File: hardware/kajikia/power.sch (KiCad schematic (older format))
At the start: 80 parts, among them J39 Screw_Terminal_01x02, J40 Conn_01x01, J41 Conn_01x01, J42 Conn_01x01, J43 Conn_01x01, J44 Conn_01x01, J45 Conn_01x01, J46 Conn_01x01, J47 Conn_01x01, J48 Conn_01x01, J49 Conn_01x01, J50 Conn_01x01, J51 Conn_01x01, J52 Conn_01x01, J53 Conn_01x01, J54 Conn_01x01, J55 Conn_01x01, J56 Conn_01x01, J57 Conn_01x01, J58 Conn_01x01, J59 Conn_01x01, Q1 AON6144, U2 LM1117-3.3, U3 AOZ1284, U4 AOZ1284

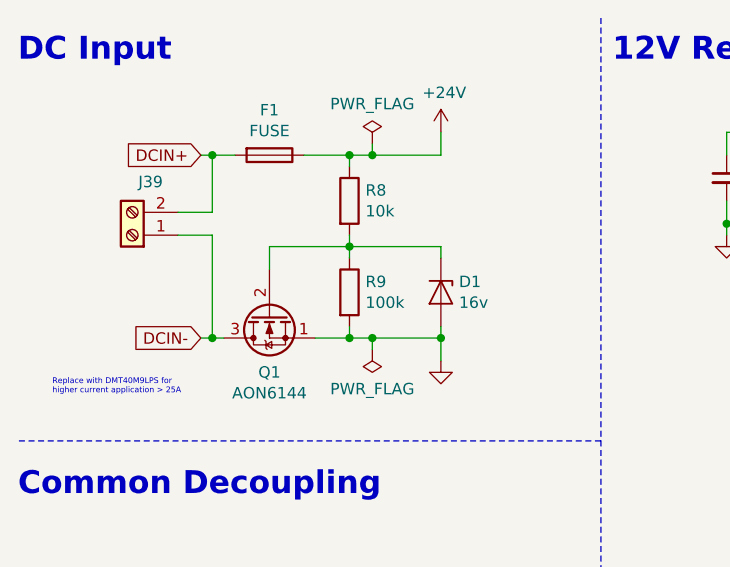
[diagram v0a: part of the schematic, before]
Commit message: fuses
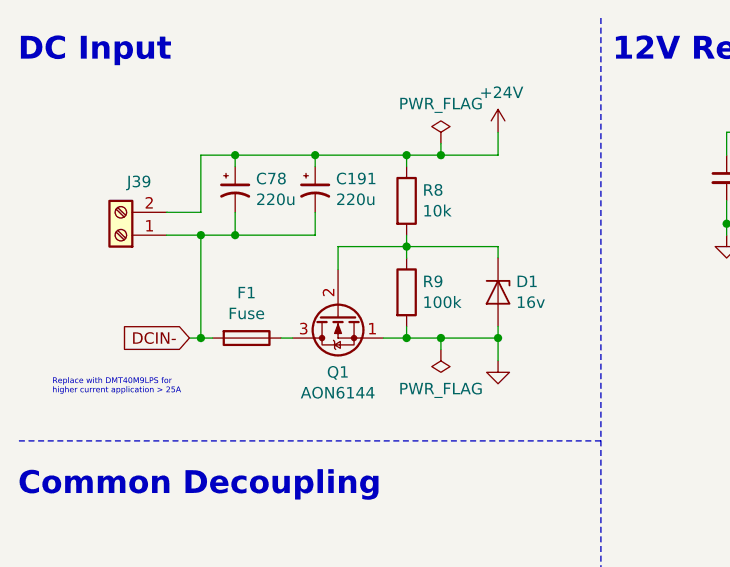
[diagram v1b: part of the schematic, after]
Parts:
- added C191, C78: 220u, Capacitor_SMD:CP_Elec_6.3x7.7, symbol Device:CP1_Small
- F1: value FUSE -> Fuse
- JP14: footprint (none) -> _Generic:Solder Jumper 2P
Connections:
- net +24V: now also J39.2 (Pin_2), C191.1, C78.1; no longer F1.1
- net DCIN-: now also F1.2, C191.2, C78.2; no longer Q1.3 (D)
- removed net DCIN+: F1.2, J39.2 (Pin_2)
- new net: F1.1, Q1.3 (D)
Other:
- moved on the sheet: D1, J39, Q1, R8, R9
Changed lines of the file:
@@
 L power:+24V #PWR017
 U 1 1 5C334E02
-P 2400 1050
-F 0 "#PWR017" H 2400 900 50  0001 C CNN
-F 1 "+24V" H 2415 1223 50  0000 C CNN
-F 2 "" H 2400 1050 50  0001 C CNN
-F 3 "" H 2400 1050 50  0001 C CNN
-	1    2400 1050
-	1    0    0    -1
-$EndComp
-Wire Wire Line
-	1250 1500 1400 1500
-Wire Wire Line
-	1400 1500 1400 1950
-Wire Wire Line
-	1250 1400 1400 1400
-Wire Wire Line
-	1400 1400 1400 1150
+P 2650 1050
+F 0 "#PWR017" H 2650 900 50  0001 C CNN
+F 1 "+24V" H 2665 1223 50  0000 C CNN
+F 2 "" H 2650 1050 50  0001 C CNN
+F 3 "" H 2650 1050 50  0001 C CNN
+	1    2650 1050
+	1    0    0    -1
+$EndComp
+Wire Wire Line
+	1200 1500 1350 1500
+Wire Wire Line
+	1200 1400 1350 1400
 $Comp
 L #Power:GND #PWR018
 U 1 1 5C34B6E8
-P 2400 2050
-F 0 "#PWR018" H 2400 1800 50  0001 C CNN
-F 1 "GND" H 2400 1900 50  0001 C CNN
-F 2 "" H 2400 2050 50  0001 C CNN
-F 3 "" H 2400 2050 50  0001 C CNN
-	1    2400 2050
-	1    0    0    -1
-$EndComp
-Wire Wire Line
-	2400 1950 2400 2050
-Wire Wire Line
-	2400 1050 2400 1150
-Wire Wire Line
-	1400 1150 1500 1150
-$Comp
-L Device:Fuse F1
-U 1 1 5C35C7B9
-P 1650 1150
-F 0 "F1" V 1453 1150 50  0000 C CNN
-F 1 "FUSE" V 1544 1150 50  0000 C CNN
-F 2 "_Generic:SMD_Fuseholder" V 1580 1150 50  0001 C CNN
-F 3 "~" H 1650 1150 50  0001 C CNN
-	1    1650 1150
-	0    1    1    0
-$EndComp
+P 2650 2050
+F 0 "#PWR018" H 2650 1800 50  0001 C CNN
+F 1 "GND" H 2650 1900 50  0001 C CNN
+F 2 "" H 2650 2050 50  0001 C CNN
+F 3 "" H 2650 2050 50  0001 C CNN
+	1    2650 2050
+	1    0    0    -1
+$EndComp
+Wire Wire Line
+	2650 1950 2650 2050
+Wire Wire Line
+	2650 1050 2650 1150
 $Comp
 L power:+12V #PWR034
@@
 F 0 "JP14" H 8300 1363 50  0000 C CNN
 F 1 "SolderJumper_2_Open" H 8300 1250 50  0001 C CNN
-F 2 "" H 8300 1250 50  0001 C CNN
+F 2 "_Generic:Solder Jumper 2P" H 8300 1250 50  0001 C CNN
 F 3 "~" H 8300 1250 50  0001 C CNN
 	1    8300 1250
@@
 Power LED
 Wire Wire Line
-	1400 1950 1450 1950
+	1350 1950 1400 1950
 $Comp
 L Device:Q_NMOS_SGD Q1
 U 1 1 5C3AA6BF
-P 1650 1850
-F 0 "Q1" V 1900 1850 50  0000 C CNN
-F 1 "AON6144" V 1991 1850 50  0000 C CNN
-F 2 "_Generic:DFN5x6-8" H 1850 1950 50  0001 C CNN
-F 3 "~" H 1650 1850 50  0001 C CNN
-	1    1650 1850
+P 1950 1850
+F 0 "Q1" V 2200 1850 50  0000 C CNN
+F 1 "AON6144" V 2291 1850 50  0000 C CNN
+F 2 "_Generic:DFN5x6-8" H 2150 1950 50  0001 C CNN
+F 3 "~" H 1950 1850 50  0001 C CNN
+	1    1950 1850
 	0    -1   1    0
 $EndComp
 Wire Wire Line
-	1850 1950 2000 1950
+	2150 1950 2250 1950
 $Comp
 L Device:R R8
 U 1 1 5C407302
-P 2000 1350
-F 0 "R8" H 2070 1396 50  0000 L CNN
-F 1 "10k" H 2070 1305 50  0000 L CNN
-F 2 "_Generic:0603_RES" V 1930 1350 50  0001 C CNN
-F 3 "~" H 2000 1350 50  0001 C CNN
-	1    2000 1350
+P 2250 1350
+F 0 "R8" H 2320 1396 50  0000 L CNN
+F 1 "10k" H 2320 1305 50  0000 L CNN
+F 2 "_Generic:0603_RES" V 2180 1350 50  0001 C CNN
+F 3 "~" H 2250 1350 50  0001 C CNN
+	1    2250 1350
 	1    0    0    -1
 $EndComp
@@
 L Device:D_Zener D1
 U 1 1 5C407892
-P 2400 1750
-F 0 "D1" V 2354 1829 50  0000 L CNN
-F 1 "16v" V 2445 1829 50  0000 L CNN
-F 2 "_Generic:SOD-523_DIODE" H 2400 1750 50  0001 C CNN
-F 3 "~" H 2400 1750 50  0001 C CNN
-	1    2400 1750
+P 2650 1750
+F 0 "D1" V 2604 1829 50  0000 L CNN
+F 1 "16v" V 2695 1829 50  0000 L CNN
+F 2 "_Generic:SOD-523_DIODE" H 2650 1750 50  0001 C CNN
+F 3 "~" H 2650 1750 50  0001 C CNN
+	1    2650 1750
 	0    1    1    0
 $EndComp
 Wire Wire Line
-	2400 1600 2400 1550
-Wire Wire Line
-	2400 1550 2000 1550
-Wire Wire Line
-	1650 1550 1650 1650
-Wire Wire Line
-	2000 1550 2000 1500
-Wire Wire Line
-	2400 1900 2400 1950
-Connection ~ 2400 1950
+	2650 1600 2650 1550
+Wire Wire Line
+	2650 1550 2250 1550
+Wire Wire Line
+	1950 1550 1950 1650
+Wire Wire Line
+	2250 1550 2250 1500
+Wire Wire Line
+	2650 1900 2650 1950
+Connection ~ 2650 1950
 $Comp
 L Device:R R9
 U 1 1 5C479547
-P 2000 1750
-F 0 "R9" H 2070 1796 50  0000 L CNN
-F 1 "100k" H 2070 1705 50  0000 L CNN
-F 2 "_Generic:0603_RES" V 1930 1750 50  0001 C CNN
-F 3 "~" H 2000 1750 50  0001 C CNN
-	1    2000 1750
-	1    0    0    -1
-$EndComp
-Wire Wire Line
-	2000 1900 2000 1950
-Connection ~ 2000 1950
-Wire Wire Line
-	2000 1950 2100 1950
-Wire Wire Line
-	2000 1600 2000 1550
-Connection ~ 2000 1550
-Wire Wire Line
-	2000 1550 1650 1550
+P 2250 1750
+F 0 "R9" H 2320 1796 50  0000 L CNN
+F 1 "100k" H 2320 1705 50  0000 L CNN
+F 2 "_Generic:0603_RES" V 2180 1750 50  0001 C CNN
+F 3 "~" H 2250 1750 50  0001 C CNN
+	1    2250 1750
+	1    0    0    -1
+$EndComp
+Wire Wire Line
+	2250 1900 2250 1950
+Connection ~ 2250 1950
+Wire Wire Line
+	2250 1600 2250 1550
+Connection ~ 2250 1550
+Wire Wire Line
+	2250 1550 1950 1550
 Text Notes 700  2200 0    25   ~ 0
 Replace with DMT40M9LPS for\nhigher current application > 25A
@@
 L power:PWR_FLAG #FLG07
 U 1 1 5C5382D5
-P 2100 2000
-F 0 "#FLG07" H 2100 2075 50  0001 C CNN
-F 1 "PWR_FLAG" H 2100 2173 50  0000 C CNN
-F 2 "" H 2100 2000 50  0001 C CNN
-F 3 "~" H 2100 2000 50  0001 C CNN
-	1    2100 2000
+P 2400 2000
+F 0 "#FLG07" H 2400 2075 50  0001 C CNN
+F 1 "PWR_FLAG" H 2400 2173 50  0000 C CNN
+F 2 "" H 2400 2000 50  0001 C CNN
+F 3 "~" H 2400 2000 50  0001 C CNN
+	1    2400 2000
 	-1   0    0    1
 $EndComp
 Wire Wire Line
-	2100 2000 2100 1950
-Connection ~ 2100 1950
-Wire Wire Line
-	2100 1950 2400 1950
+	2400 2000 2400 1950
 $Comp
 L power:PWR_FLAG #FLG06
 U 1 1 5C5499F4
-P 2100 1100
-F 0 "#FLG06" H 2100 1175 50  0001 C CNN
-F 1 "PWR_FLAG" H 2100 1274 50  0000 C CNN
-F 2 "" H 2100 1100 50  0001 C CNN
-F 3 "~" H 2100 1100 50  0001 C CNN
-	1    2100 1100
-	1    0    0    -1
-$EndComp
-Wire Wire Line
-	2100 1100 2100 1150
-Connection ~ 2100 1150
-Wire Wire Line
-	2100 1150 2400 1150
-Wire Wire Line
-	2000 1200 2000 1150
-Connection ~ 2000 1150
-Wire Wire Line
-	2000 1150 2100 1150
-Wire Wire Line
-	1800 1150 2000 1150
+P 2400 1100
+F 0 "#FLG06" H 2400 1175 50  0001 C CNN
+F 1 "PWR_FLAG" H 2400 1274 50  0000 C CNN
+F 2 "" H 2400 1100 50  0001 C CNN
+F 3 "~" H 2400 1100 50  0001 C CNN
+	1    2400 1100
+	1    0    0    -1
+$EndComp
+Wire Wire Line
+	2400 1100 2400 1150
+Wire Wire Line
+	2250 1200 2250 1150
+Connection ~ 2250 1150
 $Comp
 L Connector:Screw_Terminal_01x02 J39
 U 1 1 5C365574
-P 1050 1500
-F 0 "J39" H 970 1267 50  0000 C CNN
-F 1 "Screw_Terminal_01x02" H 970 1266 50  0001 C CNN
-F 2 "_Generic:KF635-2P" H 1050 1500 50  0001 C CNN
-F 3 "~" H 1050 1500 50  0001 C CNN
-	1    1050 1500
+P 1000 1500
+F 0 "J39" H 920 1267 50  0000 C CNN
+F 1 "Screw_Terminal_01x02" H 920 1266 50  0001 C CNN
+F 2 "_Generic:KF635-2P" H 1000 1500 50  0001 C CNN
+F 3 "~" H 1000 1500 50  0001 C CNN
+	1    1000 1500
 	-1   0    0    1
 $EndComp
@@
 Wire Wire Line
 	8400 6300 8600 6300
-Text GLabel 1350 1150 0    50   Input ~ 0
-DCIN+
-Wire Wire Line
-	1400 1150 1350 1150
-Connection ~ 1400 1150
-Text GLabel 1350 1950 0    50   Input ~ 0
+Text GLabel 1300 1950 0    50   Input ~ 0
 DCIN-
 Wire Wire Line
-	1400 1950 1350 1950
-Connection ~ 1400 1950
+	1350 1950 1300 1950
+Connection ~ 1350 1950
+Wire Wire Line
+	1350 1150 1500 1150
+$Comp
+L Device:Fuse F1
+U 1 1 5C420B0B
+P 1550 1950
+F 0 "F1" V 1353 1950 50  0000 C CNN
+F 1 "Fuse" V 1444 1950 50  0000 C CNN
+F 2 "_Generic:SMD_Fuseholder" V 1480 1950 50  0001 C CNN
+F 3 "~" H 1550 1950 50  0001 C CNN
+	1    1550 1950
+	0    1    1    0
+$EndComp
+Wire Wire Line
+	1700 1950 1750 1950
+Connection ~ 2400 1950
+Wire Wire Line
+	2400 1950 2650 1950
+Wire Wire Line
+	2250 1950 2400 1950
+Connection ~ 2400 1150
+Wire Wire Line
+	2400 1150 2650 1150
+Wire Wire Line
+	2250 1150 2400 1150
+$Comp
+L Device:CP1_Small C78
+U 1 1 5C8D0CF9
+P 1500 1300
+F 0 "C78" H 1591 1346 50  0000 L CNN
+F 1 "220u" H 1591 1255 50  0000 L CNN
+F 2 "Capacitor_SMD:CP_Elec_6.3x7.7" H 1500 1300 50  0001 C CNN
+F 3 "~" H 1500 1300 50  0001 C CNN
+	1    1500 1300
+	1    0    0    -1
+$EndComp
+Wire Wire Line
+	1500 1400 1500 1500
+Wire Wire Line
+	1500 1500 1350 1500
+Connection ~ 1350 1500
+Wire Wire Line
+	1350 1500 1350 1950
+$Comp
+L Device:CP1_Small C191
+U 1 1 5C910F5C
+P 1850 1300
+F 0 "C191" H 1941 1346 50  0000 L CNN
+F 1 "220u" H 1941 1255 50  0000 L CNN
+F 2 "Capacitor_SMD:CP_Elec_6.3x7.7" H 1850 1300 50  0001 C CNN
+F 3 "~" H 1850 1300 50  0001 C CNN
+	1    1850 1300
+	1    0    0    -1
+$EndComp
+Wire Wire Line
+	1850 1400 1850 1500
+Wire Wire Line
+	1500 1500 1850 1500
+Connection ~ 1500 1500
+Wire Wire Line
+	1350 1150 1350 1400
+Wire Wire Line
+	1500 1150 1500 1200
+Connection ~ 1500 1150
+Wire Wire Line
+	1500 1150 1850 1150
+Wire Wire Line
+	1850 1150 1850 1200
+Connection ~ 1850 1150
+Wire Wire Line
+	1850 1150 2250 1150
 $EndSCHEMATC
